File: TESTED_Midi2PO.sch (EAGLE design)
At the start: 25 parts, among them IC1 TL071P, X1 PG203J

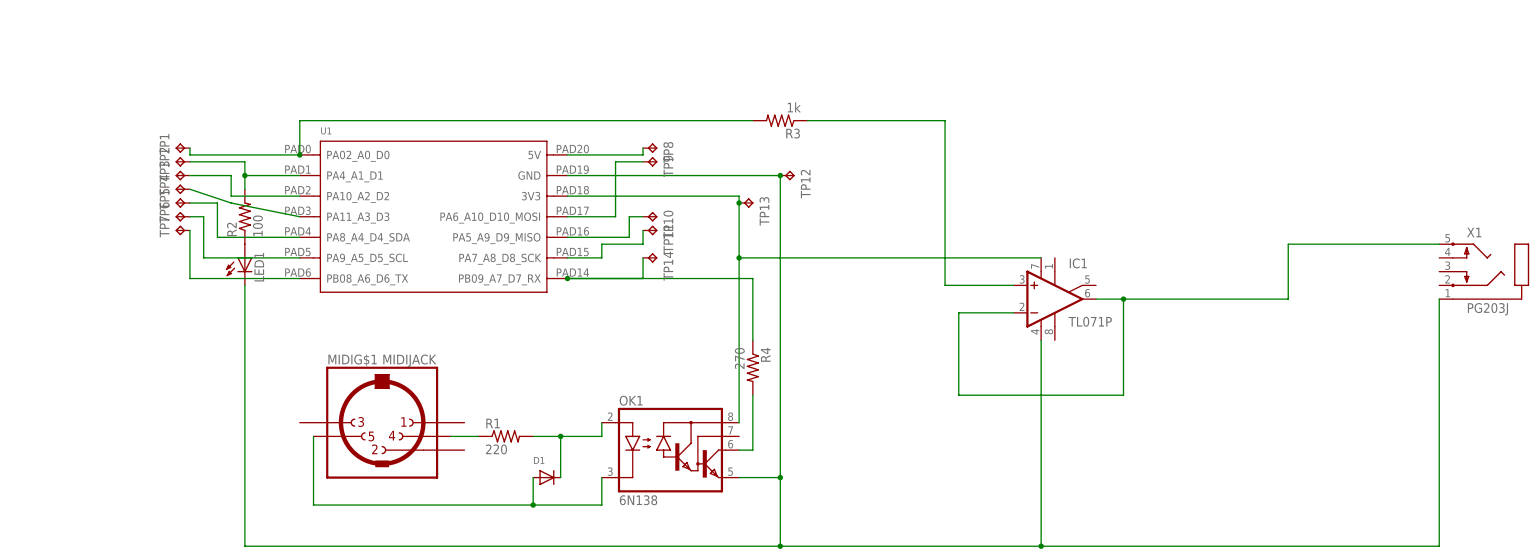
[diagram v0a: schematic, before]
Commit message: Restructured Project
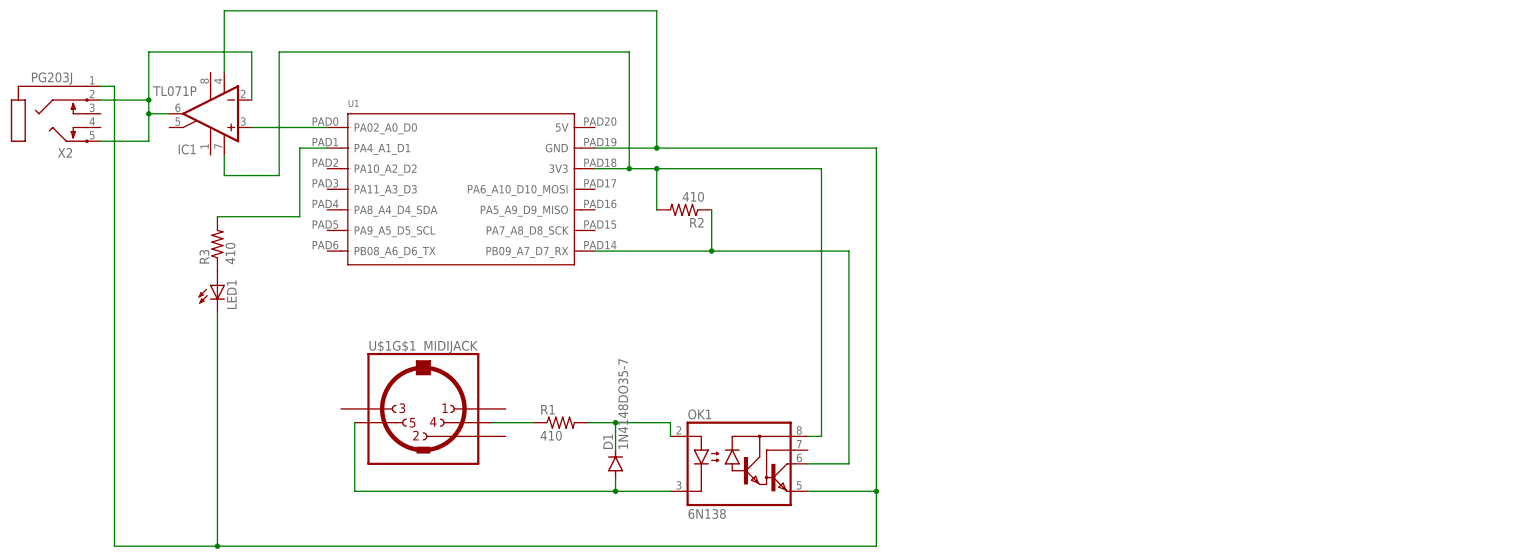
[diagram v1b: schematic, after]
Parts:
- removed MIDI: MIDIJACK, adafruit:MIDIJACK
- removed R4: 270, adafruit:R-US_0207/10
- removed TP1, TP10, TP11, TP12, TP13, TP14, TP2, TP3, TP4, TP5, TP6, TP7, TP8, TP9: TPB2,54, testpad:TPB2,54
- removed X1: PG203J, con-hirschmann:PG203J
- added U$1: MIDIJACK, adafruit:MIDIJACK
- added X2: PG203J, con-hirschmann:PG203J
- D1: value (none) -> 1N4148DO35-7; device adafruit:DIODEDO-1N4148 -> diode:1N4148DO35-7
- IC1: device linear3:TL071P -> linear:TL071P
- LED1: device adafruit:LEDSFH480 -> adafruit:LED5MM
- R1: value 220 -> 410; device adafruit:R-US_0207/10 -> adafruit:R-US_0207/9
- R2: value 100 -> 410; device adafruit:R-US_0207/10 -> adafruit:R-US_0207/9
- R3: value 1k -> 410; device adafruit:R-US_0207/10 -> adafruit:R-US_0207/9
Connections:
- removed net N$10: IC1.+IN, R3.1
- removed net N$12: TP6.TP, U1.PA9_A5_D5_SCL
- removed net N$13: TP7.TP, U1.PB08_A6_D6_TX
- removed net N$14: LED1.A, R2.1
- removed net N$15: IC1.V-, LED1.C, OK1.GND, TP12.TP, U1.GND, X1.1
- removed net N$16: R2.2, TP2.TP, U1.PA4_A1_D1
- removed net N$17: TP8.TP, U1.5V
- removed net N$18: TP9.TP, U1.PA6_A10_D10_MOSI
- removed net N$19: TP10.TP, U1.PA5_A9_D9_MISO
- removed net N$20: TP11.TP, U1.PA7_A8_D8_SCK
- removed net N$21: OK1.VO, R4.2
- net N$11: now also X2.2, X2.5; no longer X1.5
- net N$2: now also U$1G$1.4; no longer MIDIG$1.4
- net N$3: now also U$1G$1.5; no longer MIDIG$1.5
- net N$4: now also IC1.V-, LED1.C, OK1.GND, U1.GND, X2.1; no longer TP3.TP, U1.PA10_A2_D2
- net N$5: now also OK1.VO, R2.1, U1.PB09_A7_D7_RX; no longer IC1.V+, OK1.VCC, TP13.TP, U1.3V3
- net N$6: now also IC1.V+, OK1.VCC, R2.2, U1.3V3; no longer R4.1, TP14.TP, U1.PB09_A7_D7_RX
- net N$7: now also IC1.+IN, U1.PA02_A0_D0; no longer TP4.TP, U1.PA11_A3_D3
- net N$8: now also LED1.A, R3.1; no longer R3.2, TP1.TP, U1.PA02_A0_D0
- net N$9: now also R3.2, U1.PA4_A1_D1; no longer TP5.TP, U1.PA8_A4_D4_SDA
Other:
- moved on the sheet: IC1, LED1, OK1, R1, R2, R3, U1
